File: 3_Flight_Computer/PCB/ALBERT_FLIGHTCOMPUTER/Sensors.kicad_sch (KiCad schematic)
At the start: 11 parts, among them IC1 BMP390, U3 BMI088, U4 LSM6DSLTR, U5 BMM150

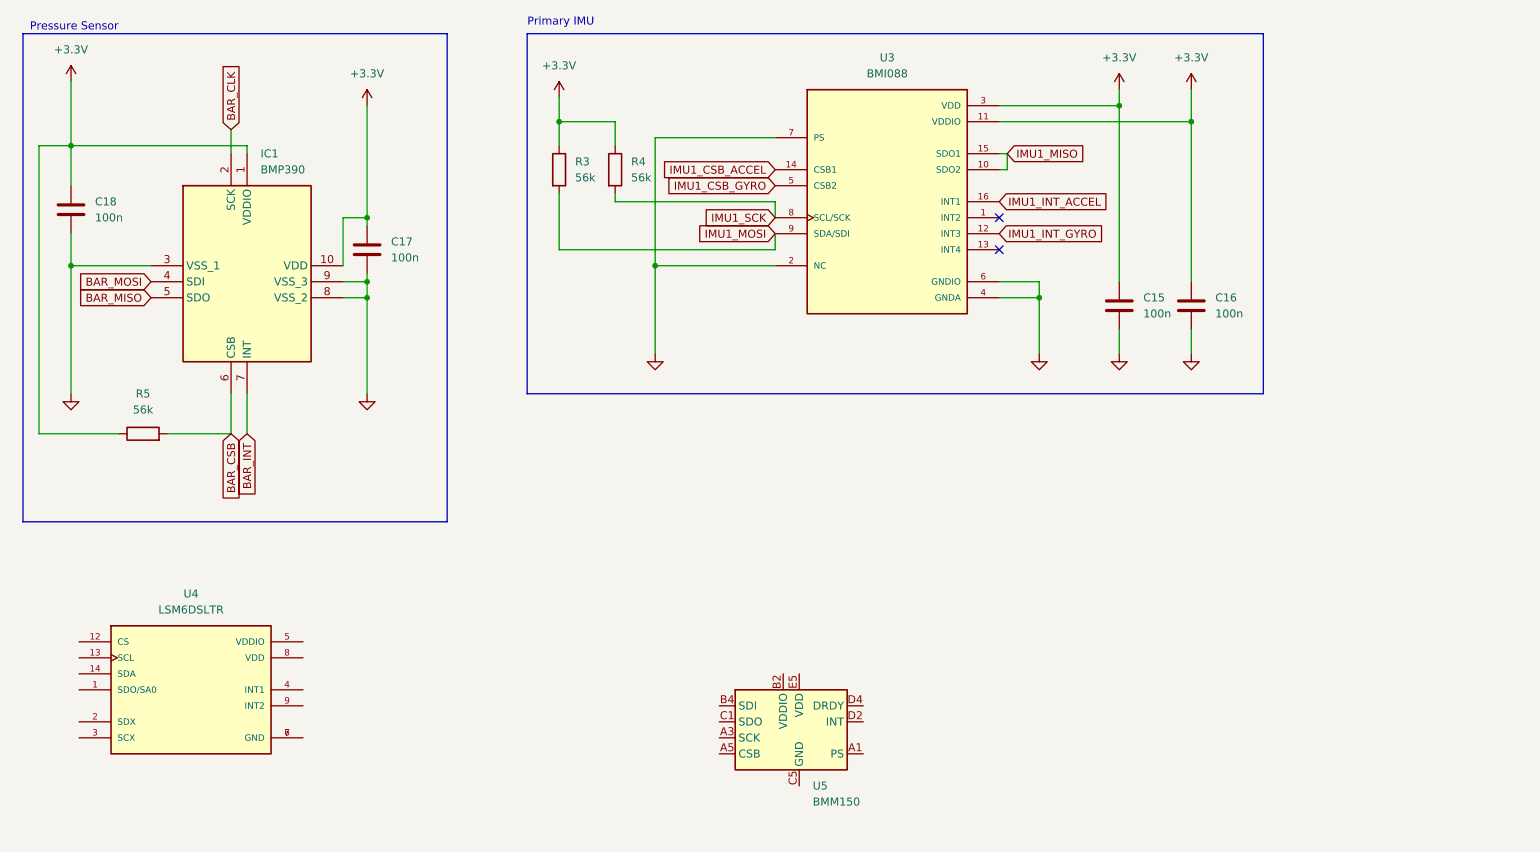
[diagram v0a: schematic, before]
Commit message: update
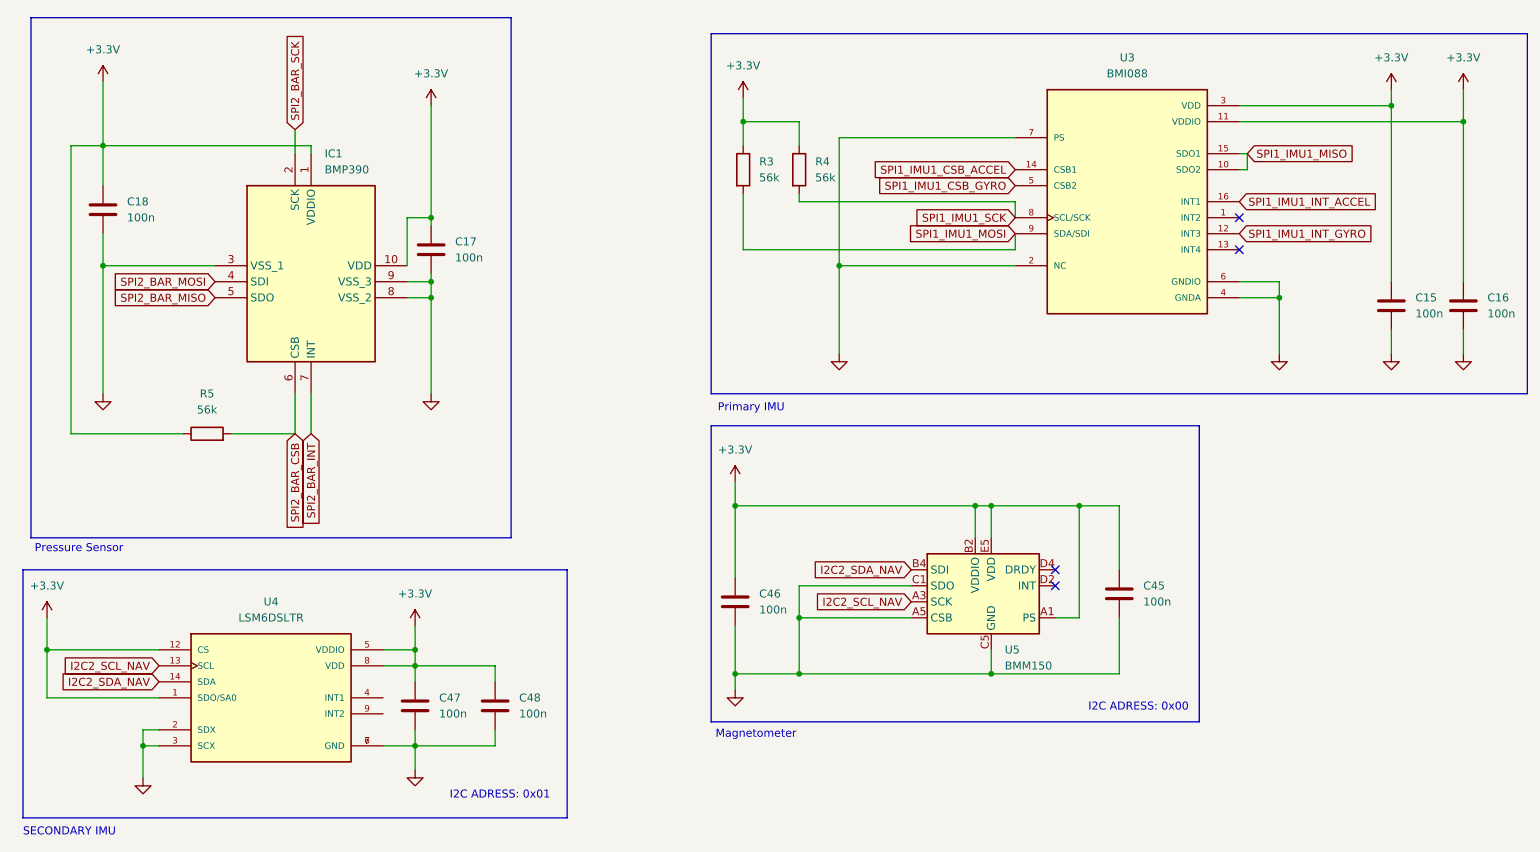
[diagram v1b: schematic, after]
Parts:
- added C45, C46, C47, C48: 100n, symbol Device:C
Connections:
- net +3.3V: now also U4.1 (SDO/SA0), U4.12 (CS), U4.5 (VDDIO), U4.8 (VDD), U5.A1 (PS), U5.B2 (VDDIO), U5.E5 (VDD), C45.1, C46.1, C47.1, C48.1
- net GND: now also U4.2 (SDX), U4.3 (SCX), U4.6 (GND), U4.7 (GND), U5.A5 (CSB), U5.C1 (SDO), U5.C5 (GND), U5.E1 (GND), U5.E3 (GND), C45.2, C46.2, C47.2, C48.2
- net I2C2_SCL_NAV: now reaches U4.13 (SCL)
- net I2C2_SCL_NAV: now also U5.A3 (SCK)
- net I2C2_SDA_NAV: now reaches U4.14 (SDA)
- net I2C2_SDA_NAV: now also U5.B4 (SDI)
- net BAR_CLK renamed SPI2_BAR_SCK
- net BAR_CSB renamed SPI2_BAR_CSB
- net BAR_INT renamed SPI2_BAR_INT
- net BAR_MISO renamed SPI2_BAR_MISO
- net BAR_MOSI renamed SPI2_BAR_MOSI
- net IMU1_CSB_ACCEL renamed SPI1_IMU1_CSB_ACCEL
- net IMU1_CSB_GYRO renamed SPI1_IMU1_CSB_GYRO
- net IMU1_INT_ACCEL renamed SPI1_IMU1_INT_ACCEL
- net IMU1_INT_GYRO renamed SPI1_IMU1_INT_GYRO
- net IMU1_MISO renamed SPI1_IMU1_MISO
- net IMU1_MOSI renamed SPI1_IMU1_MOSI
- net IMU1_SCK renamed SPI1_IMU1_SCK
- no-connect marks 2 -> 4
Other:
- note added: "I2C ADRESS: 0x00"
- note added: "I2C ADRESS: 0x01"
- note added: "Magnetometer"
- note added: "SECONDARY IMU"
- title: (none) -> Sensors and Peripherals
- moved on the sheet: C15, C16, C17, C18, IC1, R3, R4, R5, U3, U4, U5
